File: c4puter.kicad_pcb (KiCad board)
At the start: 6 copper layers, 200 x 200 mm, 154 parts, among them J7 19V 3A, J8 DEBUG, Q1 DMN3016LDN, U1 ADP5054, U2 INA199, U3 AOZ1037, U5 INA199, U6 INA199, U8 INA199, U9 TLV70225DBV

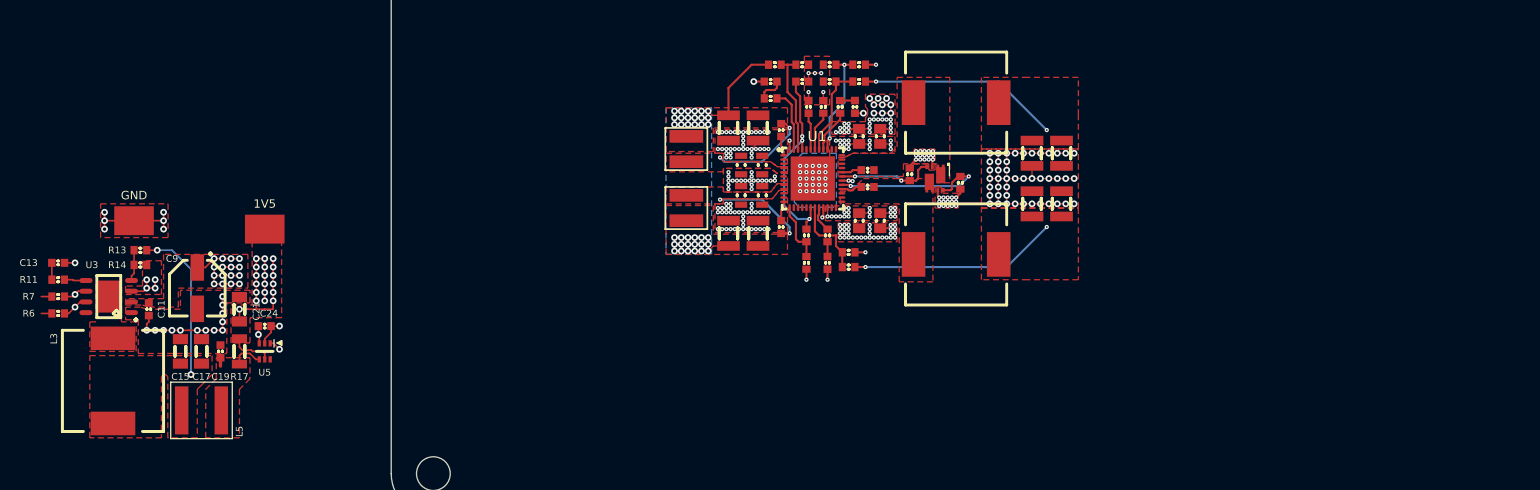
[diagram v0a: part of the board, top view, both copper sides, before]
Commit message: More power supply work
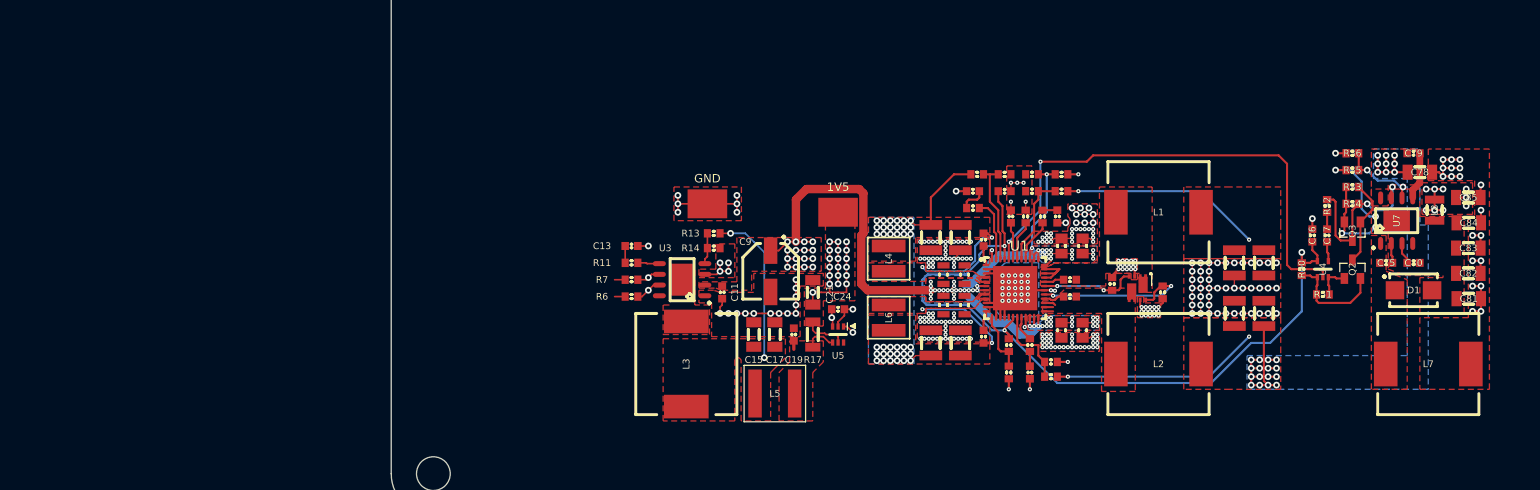
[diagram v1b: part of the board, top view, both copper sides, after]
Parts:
- added C75: 100n, IPC7351-Nominal:CAPC1608X55, F.Cu at (118.0, 170.0)
- added C76: 100n, IPC7351-Nominal:CAPC1608X55, F.Cu at (109.2, 166.8)
- added C77: 2n2, IPC7351-Nominal:CAPC1608X55, F.Cu at (111.0, 166.8)
- added C78: 22u, IPC7351-Nominal:CAPC3216X70, F.Cu at (122.0, 159.2)
- added C79: 100n, IPC7351-Nominal:CAPC1608X55, F.Cu at (121.2, 157.0)
- added C80: 1u, IPC7351-Nominal:CAPC1608X55, F.Cu at (121.2, 170.0)
- added C81: 22u, IPC7351-Nominal:CAPC3216X70, F.Cu at (127.8, 174.2)
- added C82: 22u, IPC7351-Nominal:CAPC3216X70, F.Cu at (127.8, 171.2)
- added C83: 22u, IPC7351-Nominal:CAPC3216X70, F.Cu at (127.8, 168.2)
- added C84: 22u, IPC7351-Nominal:CAPC3216X70, F.Cu at (127.8, 165.2)
- added C85: 22u, IPC7351-Nominal:CAPC3216X70, F.Cu at (127.8, 162.2)
- added D1: MBRS360B, IPC7351-Nominal:DIOM5436X244, F.Cu at (121.2, 173.2)
- added L7: 22u, manuf:BOURNS-SRR1210, F.Cu at (123.0, 182.0)
- added L8: 2u2, IPC7351-Nominal:INDC2520X220, F.Cu at (123.8, 163.8)
- added Q2: BSS84, smd-semi:SOT-23, F.Cu at (114.0, 170.8)
- added Q3: 2N7002, smd-semi:SOT-23, F.Cu at (114.0, 166.2)
- added R50: 10k, IPC7351-Nominal:RESC1608X50, F.Cu at (108.0, 170.8)
- added R51: 20k, IPC7351-Nominal:RESC1608X50, F.Cu at (110.5, 173.8)
- added R52: 1k, IPC7351-Nominal:RESC1608X50, F.Cu at (111.0, 163.2)
- added R53: 100k, IPC7351-Nominal:RESC1608X50, F.Cu at (114.0, 161.0)
- added R54: 100k, IPC7351-Nominal:RESC1608X50, F.Cu at (114.0, 163.0)
- added R55: 10k, IPC7351-Nominal:RESC1608X50, F.Cu at (114.0, 159.0)
- added R56: 10k, IPC7351-Nominal:RESC1608X50, F.Cu at (114.0, 157.0)
- added U4: 74HCT1G02, smd-semi:SC-70-5, F.Cu at (110.5, 170.8)
- added U7: RT7258GSP, IPC7351-Nominal:SOIC127P600X170-9, F.Cu at (119.2, 165.0)
- moved C11 68.0 mm to (39.2, 173.5)
- moved C13 68.0 mm to (28.5, 168.0)
- moved C15 68.0 mm to (43.0, 178.5)
- moved C17 68.0 mm to (45.5, 178.5)
- moved C19 68.0 mm to (47.8, 178.5)
- moved C21 68.0 mm to (50.0, 173.5)
- moved C24 68.0 mm to (53.0, 175.5)
- moved C9 68.0 mm to (45.0, 171.0)
- moved L3 68.0 mm to (35.0, 182.0)
- moved L5 68.0 mm to (45.5, 185.5)
- moved R11 68.0 mm to (28.5, 170.0)
- moved R13 68.0 mm to (38.2, 166.5)
- moved R14 68.0 mm to (38.2, 168.2)
- moved R17 68.0 mm to (50.0, 178.5)
- moved R6 68.0 mm to (28.5, 174.0)
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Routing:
- net /Power/VREG: track 23.9 -> 91.2 mm
- net +12: track 51.0 -> 113.2 mm
- net Net-(U1-Pad44): track 0.00 -> 60.3 mm, vias 0 -> 2
- net GND: track 278.8 -> 335.8 mm, vias 339 -> 360
- net P5V: track 24.7 -> 56.5 mm, vias 2 -> 27
- net /Power/UNFN12: track 0.00 -> 25.8 mm, vias 0 -> 4
- net Net-(Q3-Pad3): track 0.00 -> 20.1 mm, vias 0 -> 2
- net ENN12#: track 0.00 -> 12.3 mm
- net Net-(Q2-Pad3): track 0.00 -> 10.3 mm
- net N5V: track 0.00 -> 9.70 mm, vias 0 -> 9
- net Net-(R55-Pad1): track 0.00 -> 9.43 mm, vias 0 -> 2
- net /Power/SW3V: track 0.00 -> 5.67 mm
- net /Power/SW5V: track 0.00 -> 3.50 mm
- net /Power/SWA1V2: track 11.8 -> 14.6 mm
- net Net-(C80-Pad1): track 0.00 -> 2.55 mm
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- added copper zone on B.Cu, net +12
- added copper zone on F.Cu, net /Power/SWN12
- added copper zone on F.Cu, net /Power/UNFN12
- added copper zone on F.Cu, net N5V
- added copper zone on B.Cu, net P5V

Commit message: Uh, more misc work.
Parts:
- removed C10: 10u, IPC7351-Nominal:CAPC2012X70
- removed C11, C19, C22, C23, C24, C25, C26, C27, C32, C75, C76, C79: 100n, IPC7351-Nominal:CAPC1608X55
- removed C12, C16, C30, C31, C55, C56, C57, C59: 100u, IPC7351-Nominal:CAPC3225X88
- removed C13: 220p, IPC7351-Nominal:CAPC1608X55
- removed C14: 4n5, IPC7351-Nominal:CAPC1608X55
- removed C15, C17, C21, C78, C81, C82, C83, C84, C85: 22u, IPC7351-Nominal:CAPC3216X70
- removed C18: 3n6, IPC7351-Nominal:CAPC1608X55
- removed C20: 4n9, IPC7351-Nominal:CAPC1608X55
- removed C28, C29, C80: 1u, IPC7351-Nominal:CAPC1608X55
- removed C33, C34: 2u2, IPC7351-Nominal:CAPC1608X55
- removed C77: 2n2, IPC7351-Nominal:CAPC1608X55
- removed C9: 22u(P), IPC7351-Nominal:CAPAE660X570
- removed D1: MBRS360B, IPC7351-Nominal:DIOM5436X244
- removed L1, L2, L3: 4u7, manuf:BOURNS-SRR1210
- removed L4, L6: 6u8, manuf:BOURNS-SRN5040
- removed L5: 2u2, manuf:MURATA-DG6050C
- removed L7: 22u, manuf:BOURNS-SRR1210
- removed L8: 2u2, IPC7351-Nominal:INDC2520X220
- removed R56: 10k, IPC7351-Nominal:RESC1608X50
- removed TP3: 1V5, manuf:TESTPOINT-KEYSTONE-5018
- removed TP5: 2V5, manuf:TESTPOINT-KEYSTONE-5018
- removed TP6, TP7, TP8: GND, manuf:TESTPOINT-KEYSTONE-5018
- removed U2, U5, U6, U8: INA199, smd-semi:SC-70-6
- removed U3: AOZ1037, IPC7351-Nominal:SOIC127P600X175-9
- removed U4: 74HCT1G02, smd-semi:SC-70-5
- removed U7: RT7258GSP, IPC7351-Nominal:SOIC127P600X170-9
- removed U9: TLV70225DBV, smd-semi:SOT-23-5
- added DS1: PCI_P12(R), smd-semi:LED-0603, F.Cu at (86.5, 164.0)
- added DS10: BRG_P3V3(R), smd-semi:LED-0603, F.Cu at (96.5, 169.0)
- added DS11: CPU_P3V3(R), smd-semi:LED-0603, F.Cu at (96.5, 179.0)
- added DS12: AUX_P3V3(R), smd-semi:LED-0603, F.Cu at (96.5, 184.0)
- added DS13: SBY_P3V3(R), smd-semi:LED-0603, F.Cu at (96.5, 189.0)
- added DS14: PCI_P3V3(G), smd-semi:LED-0603, F.Cu at (98.5, 164.0)
- added DS15: BRG_P3V3(G), smd-semi:LED-0603, F.Cu at (98.5, 169.0)
- added DS16: CPU_P3V3(G), smd-semi:LED-0603, F.Cu at (98.5, 179.0)
- added DS17: AUX_P3V3(G), smd-semi:LED-0603, F.Cu at (98.5, 184.0)
- added DS18: SBY_P3V3(G), smd-semi:LED-0603, F.Cu at (98.5, 189.0)
- added DS19: BRG_P2V5(R), smd-semi:LED-0603, F.Cu at (101.5, 169.0)
- added DS2: PCI_P12(G), smd-semi:LED-0603, F.Cu at (88.5, 164.0)
- added DS20: CPU_P2V5(R), smd-semi:LED-0603, F.Cu at (101.5, 179.0)
- added DS21: BRG_P2V5(G), smd-semi:LED-0603, F.Cu at (103.5, 169.0)
- added DS22: CPU_P2V5(G), smd-semi:LED-0603, F.Cu at (103.5, 179.0)
- added DS23: BRG_P1V5(R), smd-semi:LED-0603, F.Cu at (106.5, 169.0)
- added DS24: MEM_P1V5(R), smd-semi:LED-0603, F.Cu at (106.5, 174.0)
- added DS25: CPU_P1V5(R), smd-semi:LED-0603, F.Cu at (106.5, 179.0)
- added DS26: BRG_P1V5(G), smd-semi:LED-0603, F.Cu at (108.5, 169.0)
- added DS27: MEM_P1V5(G), smd-semi:LED-0603, F.Cu at (108.5, 174.0)
- added DS28: CPU_P1V5(G), smd-semi:LED-0603, F.Cu at (108.5, 179.0)
- added DS29: BRG_P1V2(R), smd-semi:LED-0603, F.Cu at (111.5, 169.0)
- added DS3: PCI_P5(R), smd-semi:LED-0603, F.Cu at (91.5, 164.0)
- added DS30: CPU_P1V2(R), smd-semi:LED-0603, F.Cu at (111.5, 179.0)
- added DS31: BRG_P1V2(G), smd-semi:LED-0603, F.Cu at (113.5, 169.0)
- added DS32: CPU_P1V2(G), smd-semi:LED-0603, F.Cu at (113.5, 179.0)
- added DS33: PCI_N12(R), smd-semi:LED-0603, F.Cu at (116.5, 164.0)
- added DS34: MEM_PV75(R), smd-semi:LED-0603, F.Cu at (116.5, 174.0)
- added DS35: PCI_N12(G), smd-semi:LED-0603, F.Cu at (118.5, 164.0)
- added DS36: MEM_PV75(G), smd-semi:LED-0603, F.Cu at (118.5, 174.0)
- added DS37: POWER(R), smd-semi:LED-0603, F.Cu at (135.0, 164.0)
- added DS38: CARD(R), smd-semi:LED-0603, F.Cu at (135.0, 169.0)
- added DS39: BIT(R), smd-semi:LED-0603, F.Cu at (135.0, 174.0)
- added DS4: BRG_P5(R), smd-semi:LED-0603, F.Cu at (91.5, 169.0)
- added DS40: CLK(R), smd-semi:LED-0603, F.Cu at (135.0, 179.0)
- added DS41: MEM(R), smd-semi:LED-0603, F.Cu at (135.0, 184.0)
- added DS42: RUN(R), smd-semi:LED-0603, F.Cu at (135.0, 189.0)
- added DS43: POWER(G), smd-semi:LED-0603, F.Cu at (137.0, 164.0)
- added DS44: CARD(G), smd-semi:LED-0603, F.Cu at (137.0, 169.0)
- added DS45: BIT-BR(G), smd-semi:LED-0603, F.Cu at (137.0, 174.0)
- added DS46: CLK(G), smd-semi:LED-0603, F.Cu at (137.0, 179.0)
- added DS47: MEM(G), smd-semi:LED-0603, F.Cu at (137.0, 184.0)
- added DS48: RUN(G), smd-semi:LED-0603, F.Cu at (137.0, 189.0)
- added DS49: BIT-CPU0(G), smd-semi:LED-0603, F.Cu at (145.5, 174.0)
- added DS5: CPU_P5(R), smd-semi:LED-0603, F.Cu at (91.5, 179.0)
- added DS50: BIT-CPU1(G), smd-semi:LED-0603, F.Cu at (152.5, 174.0)
- added DS51: UPDOG(G), smd-semi:LED-0603, F.Cu at (151.0, 189.0)
- added DS52: UNC(R), smd-semi:LED-0603, F.Cu at (161.5, 164.0)
- added DS53: UNC(R), smd-semi:LED-0603, F.Cu at (161.5, 169.0)
- added DS54: UNC(R), smd-semi:LED-0603, F.Cu at (161.5, 174.0)
- added DS55: UNC(R), smd-semi:LED-0603, F.Cu at (161.5, 179.0)
- added DS56: UNC(R), smd-semi:LED-0603, F.Cu at (161.5, 184.0)
- added DS57: UNC(R), smd-semi:LED-0603, F.Cu at (161.5, 189.0)
- added DS58: UNC(G), smd-semi:LED-0603, F.Cu at (163.5, 164.0)
- added DS59: UNC(G), smd-semi:LED-0603, F.Cu at (163.5, 169.0)
- added DS6: PCI_P5(G), smd-semi:LED-0603, F.Cu at (93.5, 164.0)
- added DS60: UNC(G), smd-semi:LED-0603, F.Cu at (163.5, 174.0)
- added DS61: UNC(G), smd-semi:LED-0603, F.Cu at (163.5, 179.0)
- added DS62: UNC(G), smd-semi:LED-0603, F.Cu at (163.5, 184.0)
- added DS63: UNC(G), smd-semi:LED-0603, F.Cu at (163.5, 189.0)
- added DS7: BRG_P5(G), smd-semi:LED-0603, F.Cu at (93.5, 169.0)
- added DS8: CPU_P5(G), smd-semi:LED-0603, F.Cu at (93.5, 179.0)
- added DS9: PCI_P3V3(R), smd-semi:LED-0603, F.Cu at (96.5, 164.0)
- added DZ1: DRTR5V0U2SR, smd-semi:SOT-143, F.Cu at (21.2, 10.0)
- added J1: PDI, conn-100mil:CONN-100MIL-M-2x3, F.Cu at (157.0, 153.5)
- added PSU1: C4-0-PSU, conn-fci:CONN-10018783-10202TLF-PCIEx8-FCI, F.Cu at (33.0, 182.0)
- C1: value 10u -> 1u
- C2, C7: value 10u -> 100n; footprint IPC7351-Nominal:CAPC2012X70 -> IPC7351-Nominal:CAPC1005X55
- C3, C4, C5, C6: value 10u -> 390u; footprint IPC7351-Nominal:CAPC2012X70 -> pth-passive:C-ALUM-8mm
- C8: footprint IPC7351-Nominal:CAPC1608X55 -> IPC7351-Nominal:CAPC1005X55
- CPU0, CPU1: value XC6SLX16-2FTG256C -> XC6SLX25-FGG484; footprint manuf:XILINX-FT256 -> manuf:XILINX-FGG484
- LIMB1: value ATSAME70NnnA-AN -> LPC435xFET256; footprint IPC7351-Nominal:QFP50P1600X1600X160-100 -> smd-semi:BGA100P1700X1700-256
- Q1: value DMN3016LDN -> AOD4189; footprint manuf:DIODES-V-DFN3030-8 -> smd-semi:TO-252
- Q2: value BSS84 -> AOD4189; footprint smd-semi:SOT-23 -> smd-semi:TO-252
- R1: value 30k -> 100k
- R10: value 38k5 -> 750
- R11: value 10k -> 300
- R12: value 22k -> 300
- R13, R50: value 10k -> 750
- R14, R55: value 10k -> 51k
- R15: value 22k -> 750
- R16, R18, R21: value R-0603 -> 300
- R17: value 0R005 -> 51k; footprint IPC7351-Nominal:RESC3216X60 -> IPC7351-Nominal:RESC1608X50
- R19, R20: value R-0603 -> 750
- R2: value 100k -> 330k
- R22: value R-0603 -> 51k
- R3: value 10k -> 100k
- R4: value 500k -> 10k
- R5: value 200k -> 750
- R51: value 20k -> 750
- R52: value 1k -> 51k
- R53, R54, R6: value 100k -> 300
- R7: value 100k -> 51k
- R8: value 8k6 -> 51k
- R9: value 7k8 -> 51k
- U1: value ADP5054 -> ATXMEGA8E5-MU; footprint IPC7351-Nominal:QFN50P700X700X80-49 -> IPC7351-Nominal:QFN50P500X500X100-33
- moved Q3 175.1 mm to (43.5, 6.00), turned to 90 degrees
- moved R4 170.9 mm to (43.5, 11.5), turned to 180 degrees
- moved R11 162.1 mm to (190.0, 155.5), turned to 90 degrees
- moved R6 154.2 mm to (181.0, 151.5), turned to 270 degrees
- moved R3 153.5 mm to (43.5, 9.50), turned to 180 degrees
- moved R13 151.5 mm to (189.0, 151.5), turned to 90 degrees
- moved R7 123.9 mm to (151.0, 153.5), turned to 270 degrees
- moved C8 117.0 mm to (163.2, 149.4)
- moved R21 113.3 mm to (186.0, 155.5), turned to 90 degrees
- moved R19 112.9 mm to (187.0, 151.5), turned to 90 degrees
- moved R5 112.2 mm to (182.0, 155.5), turned to 270 degrees
- moved R16 112.2 mm to (188.0, 155.5), turned to 90 degrees
- moved R10 111.3 mm to (180.0, 155.5), turned to 90 degrees
- moved Q2 108.3 mm to (17.0, 122.5), turned to 180 degrees
- moved C7 107.3 mm to (171.6, 155.6), turned to 270 degrees
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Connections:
- C1 pad 1: +12 -> Net-(C1-Pad1)
- C1 pad 2: GND -> Net-(C1-Pad2)
- C2 pad 2: GND -> Net-(C1-Pad2)
- C7 pad 1: +12 -> GND
- C7 pad 2: GND -> SBY_P3V3
- C8 pad 1: +3.3SB -> GND
- C8 pad 2: GND -> SBY_P3V3
- CPU0 pad A15: (no net) -> Net-(CPU0-PadA15)
- CPU0 pad A16: (no net) -> Net-(CPU0-PadA16)
- CPU0 pad A3: (no net) -> Net-(CPU0-PadA3)
- CPU0 pad B11: (no net) -> Net-(CPU0-PadB11)
- CPU0 pad B15: (no net) -> Net-(CPU0-PadB15)
- CPU0 pad B16: (no net) -> Net-(CPU0-PadB16)
- CPU0 pad B4: (no net) -> Net-(CPU0-PadB4)
- CPU0 pad B5: Net-(CPU0-PadB5) -> (no net)
- CPU0 pad B7: (no net) -> Net-(CPU0-PadB7)
- CPU0 pad C12: (no net) -> Net-(CPU0-PadC12)
- CPU0 pad C14: (no net) -> Net-(CPU0-PadC14)
- CPU0 pad C15: (no net) -> Net-(CPU0-PadC15)
- CPU0 pad C16: (no net) -> Net-(CPU0-PadC16)
- CPU0 pad C4: Net-(CPU0-PadC4) -> (no net)
- CPU0 pad D10: (no net) -> Net-(CPU0-PadD10)
- CPU0 pad D13: (no net) -> Net-(CPU0-PadD13)
- CPU0 pad D14: (no net) -> Net-(CPU0-PadD14)
- CPU0 pad D15: (no net) -> Net-(CPU0-PadD15)
- CPU0 pad D5: Net-(CPU0-PadD5) -> (no net)
- CPU0 pad D7: (no net) -> Net-(CPU0-PadD7)
- CPU0 pad E10: Net-(CPU0-PadE10) -> (no net)
- CPU0 pad E11: Net-(CPU0-PadE11) -> (no net)
- CPU0 pad E12: (no net) -> Net-(CPU0-PadE12)
- CPU0 pad E13: (no net) -> Net-(CPU0-PadE13)
- CPU0 pad E14: (no net) -> Net-(CPU0-PadE14)
- CPU0 pad E16: (no net) -> Net-(CPU0-PadE16)
- CPU0 pad E6: Net-(CPU0-PadE6) -> (no net)
- CPU0 pad E7: Net-(CPU0-PadE7) -> (no net)
- CPU0 pad E8: Net-(CPU0-PadE8) -> (no net)
- CPU0 pad E9: (no net) -> Net-(CPU0-PadE9)
- CPU0 pad F10: Net-(CPU0-PadF10) -> (no net)
- CPU0 pad F12: (no net) -> Net-(CPU0-PadF12)
- CPU0 pad F13: (no net) -> Net-(CPU0-PadF13)
- CPU0 pad F14: (no net) -> Net-(CPU0-PadF14)
- CPU0 pad F15: (no net) -> Net-(CPU0-PadF15)
- CPU0 pad F7: Net-(CPU0-PadF7) -> (no net)
- CPU0 pad F9: Net-(CPU0-PadF9) -> (no net)
- CPU0 pad G10: (no net) -> Net-(CPU0-PadG10)
- CPU0 pad G13: (no net) -> Net-(CPU0-PadG13)
- CPU0 pad G14: (no net) -> Net-(CPU0-PadG14)
- CPU0 pad H12: (no net) -> Net-(CPU0-PadH12)
- CPU0 pad H13: (no net) -> Net-(CPU0-PadH13)
- CPU0 pad H14: (no net) -> Net-(CPU0-PadH14)
- CPU1 pad A15: (no net) -> Net-(CPU1-PadA15)
- CPU1 pad A16: (no net) -> Net-(CPU1-PadA16)
- CPU1 pad A3: (no net) -> Net-(CPU1-PadA3)
- CPU1 pad B11: (no net) -> Net-(CPU1-PadB11)
- CPU1 pad B15: (no net) -> Net-(CPU1-PadB15)
- CPU1 pad B16: (no net) -> Net-(CPU1-PadB16)
- CPU1 pad B4: (no net) -> Net-(CPU1-PadB4)
- CPU1 pad B5: Net-(CPU1-PadB5) -> (no net)
- CPU1 pad B7: (no net) -> Net-(CPU1-PadB7)
- CPU1 pad C12: (no net) -> Net-(CPU1-PadC12)
- CPU1 pad C14: (no net) -> Net-(CPU1-PadC14)
- CPU1 pad C15: (no net) -> Net-(CPU1-PadC15)
- CPU1 pad C16: (no net) -> Net-(CPU1-PadC16)
- CPU1 pad C4: Net-(CPU1-PadC4) -> (no net)
- CPU1 pad D10: (no net) -> Net-(CPU1-PadD10)
- CPU1 pad D13: (no net) -> Net-(CPU1-PadD13)
- CPU1 pad D14: (no net) -> Net-(CPU1-PadD14)
- CPU1 pad D15: (no net) -> Net-(CPU1-PadD15)
- CPU1 pad D5: Net-(CPU1-PadD5) -> (no net)
- CPU1 pad D7: (no net) -> Net-(CPU1-PadD7)
- CPU1 pad E10: Net-(CPU1-PadE10) -> (no net)
- CPU1 pad E11: Net-(CPU1-PadE11) -> (no net)
- CPU1 pad E12: (no net) -> Net-(CPU1-PadE12)
- CPU1 pad E13: (no net) -> Net-(CPU1-PadE13)
- CPU1 pad E14: (no net) -> Net-(CPU1-PadE14)
- CPU1 pad E16: (no net) -> Net-(CPU1-PadE16)
- CPU1 pad E6: Net-(CPU1-PadE6) -> (no net)
- CPU1 pad E7: Net-(CPU1-PadE7) -> (no net)
- CPU1 pad E8: Net-(CPU1-PadE8) -> (no net)
- CPU1 pad E9: (no net) -> Net-(CPU1-PadE9)
- CPU1 pad F10: Net-(CPU1-PadF10) -> (no net)
- CPU1 pad F12: (no net) -> Net-(CPU1-PadF12)
- CPU1 pad F13: (no net) -> Net-(CPU1-PadF13)
- CPU1 pad F14: (no net) -> Net-(CPU1-PadF14)
- CPU1 pad F15: (no net) -> Net-(CPU1-PadF15)
- CPU1 pad F7: Net-(CPU1-PadF7) -> (no net)
- CPU1 pad F9: Net-(CPU1-PadF9) -> (no net)
- CPU1 pad G10: (no net) -> Net-(CPU1-PadG10)
- CPU1 pad G13: (no net) -> Net-(CPU1-PadG13)
- CPU1 pad G14: (no net) -> Net-(CPU1-PadG14)
- CPU1 pad H12: (no net) -> Net-(CPU1-PadH12)
- CPU1 pad H13: (no net) -> Net-(CPU1-PadH13)
- CPU1 pad H14: (no net) -> Net-(CPU1-PadH14)
- J7 pad 1: V+ -> /12VIN
- J8 pad 1: Net-(J8-Pad1) -> Net-(DZ1-Pad4)
- J8 pad 2: Net-(J8-Pad2) -> /EC/USB0_D+
- J8 pad 3: Net-(J8-Pad3) -> /EC/USB0_D-
- J8 pad 5: Net-(J8-Pad5) -> GND
- J8 pad SH: Net-(J8-PadSH) -> GND
- Q1 pad 1: /Power/SW3V -> Net-(C1-Pad2)
- Q1 pad 2: GND -> Net-(C1-Pad1)
- Q1 pad 3: Net-(Q1-Pad3) -> /12VIN
- Q2 pad 1: GND -> Net-(C1-Pad2)
- Q2 pad 2: ENN12# -> Net-(C1-Pad1)
- Q2 pad 3: Net-(Q2-Pad3) -> +12
- Q3 pad 1: Net-(Q2-Pad3) -> Net-(DZ1-Pad4)
- Q3 pad 2: /Power/UNFN12 -> Net-(Q3-Pad2)
- Q3 pad 3: Net-(Q3-Pad3) -> 3V3_LIMB
- R1 pad 1: GND -> Net-(C1-Pad2)
- R1 pad 2: Net-(R1-Pad2) -> GND
- R10 pad 1: Net-(R10-Pad1) -> /Blinkenlights/COL0
- R10 pad 2: Net-(C20-Pad1) -> Net-(R10-Pad2)
- R11 pad 1: Net-(R11-Pad1) -> /Blinkenlights/COL6
- R11 pad 2: Net-(C13-Pad1) -> Net-(R11-Pad2)
- R12 pad 1: Net-(Q1-Pad3) -> /Blinkenlights/COL1
- R12 pad 2: GND -> Net-(R12-Pad2)
- R13 pad 1: Net-(R13-Pad1) -> /Blinkenlights/COL7
- R13 pad 2: /Power/RAW1V5 -> Net-(R13-Pad2)
- R14 pad 1: GND -> SBY_P3V3
- R14 pad 2: Net-(R13-Pad1) -> /Blinkenlights/ROW2
- R15 pad 1: Net-(Q1-Pad6) -> /Blinkenlights/COL2
- R15 pad 2: GND -> Net-(R15-Pad2)
- R16 pad 1: Net-(R16-Pad1) -> /Blinkenlights/COL8
- R16 pad 2: GND -> Net-(R16-Pad2)
- R17 pad 1: /Power/1V5 -> SBY_P3V3
- R17 pad 2: /Power/S+1V5 -> /Blinkenlights/ROW3
- R18 pad 1: P3V -> /Blinkenlights/COL3
- R18 pad 2: Net-(R16-Pad1) -> Net-(R18-Pad2)
- R19 pad 1: Net-(R19-Pad1) -> /Blinkenlights/COL9
- R19 pad 2: GND -> Net-(R19-Pad2)
- R2 pad 1: Net-(R2-Pad1) -> Net-(C1-Pad1)
- R2 pad 2: +12 -> Net-(C1-Pad2)
- R20 pad 1: P5V -> /Blinkenlights/COL4
- R20 pad 2: Net-(R19-Pad1) -> Net-(R20-Pad2)
- R21 pad 1: GND -> /Blinkenlights/COL10
- R22 pad 1: +1.2 -> SBY_P3V3
- R22 pad 2: Net-(R21-Pad2) -> /Blinkenlights/ROW4
- R3 pad 1: GND -> Net-(Q3-Pad2)
- R3 pad 2: Net-(R2-Pad1) -> GND
- R4 pad 1: Net-(R4-Pad1) -> /EC/USB0_VBUS
- R4 pad 2: /Power/VREG -> Net-(Q3-Pad2)
- R5 pad 1: GND -> Net-(R5-Pad1)
- R5 pad 2: Net-(R4-Pad1) -> /Blinkenlights/COL14
- R50 pad 1: /Power/VREG -> /Blinkenlights/COL5
- R50 pad 2: ENN12# -> Net-(R50-Pad2)
- R51 pad 1: ENN12# -> /Blinkenlights/COL11
- R51 pad 2: GND -> Net-(R51-Pad2)
- R52 pad 1: Net-(C77-Pad1) -> SBY_P3V3
- R52 pad 2: Net-(Q3-Pad3) -> /Blinkenlights/ROW5
- R53 pad 1: Net-(Q2-Pad3) -> /Blinkenlights/COL12
- R53 pad 2: /Power/UNFN12 -> Net-(R53-Pad2)
- R54 pad 1: Net-(Q3-Pad3) -> /Blinkenlights/COL13
- R54 pad 2: /Power/UNFN12 -> Net-(R54-Pad2)
- R55 pad 1: Net-(R55-Pad1) -> SBY_P3V3
- R55 pad 2: /Power/UNFN12 -> /Blinkenlights/ROW6
- R6 pad 1: +3.3SB -> Net-(R6-Pad1)
- R6 pad 2: /Power/PG1V5 -> /Blinkenlights/COL15
- R7 pad 1: /Power/EN1V5 -> SBY_P3V3
- R7 pad 2: GND -> Net-(J1-Pad5)
- R8 pad 1: Net-(R8-Pad1) -> SBY_P3V3
- R8 pad 2: Net-(C14-Pad1) -> /Blinkenlights/ROW0
- R9 pad 1: Net-(R9-Pad1) -> SBY_P3V3
- R9 pad 2: Net-(C18-Pad1) -> /Blinkenlights/ROW1
- U1 pad 1: Net-(C26-Pad2) -> GND
- U1 pad 10: GND -> Net-(R20-Pad2)
- U1 pad 11: GND -> Net-(R18-Pad2)
- U1 pad 12: Net-(C27-Pad2) -> Net-(R15-Pad2)
- U1 pad 13: Net-(R4-Pad1) -> Net-(R12-Pad2)
- U1 pad 14: GND -> Net-(R10-Pad2)
- U1 pad 15: GND -> /Blinkenlights/SCL
- U1 pad 16: GND -> /Blinkenlights/SDA
- U1 pad 17: Net-(U1-Pad17) -> SBY_P3V3
- U1 pad 18: /Power/VREG -> GND
- U1 pad 19: Net-(R19-Pad1) -> Net-(R6-Pad1)
- U1 pad 2: GND -> /Blinkenlights/ROW4
- U1 pad 20: Net-(R9-Pad1) -> Net-(R5-Pad1)
- U1 pad 21: Net-(U1-Pad21) -> Net-(R54-Pad2)
- U1 pad 22: +12 -> Net-(R53-Pad2)
- U1 pad 23: +12 -> Net-(R51-Pad2)
- U1 pad 24: +12 -> Net-(R21-Pad2)
- U1 pad 25: /Power/SW5V -> Net-(R19-Pad2)
- U1 pad 26: /Power/SW5V -> Net-(R16-Pad2)
- U1 pad 27: /Power/SW5V -> Net-(R13-Pad2)
- U1 pad 28: Net-(C25-Pad2) -> Net-(R11-Pad2)
- U1 pad 29: Net-(Q1-Pad6) -> /Blinkenlights/ROW7
- U1 pad 3: GND -> /Blinkenlights/ROW3
- U1 pad 30: GND -> /Blinkenlights/ROW6
- U1 pad 31: Net-(Q1-Pad3) -> /Blinkenlights/ROW5
- U1 pad 32: Net-(C22-Pad2) -> SBY_P3V3
- U1 pad 33: /Power/SW3V -> GND
- U1 pad 4: /Power/SWA1V2 -> /Blinkenlights/ROW2
- U1 pad 5: /Power/SWA1V2 -> /Blinkenlights/ROW1
- U1 pad 6: +12 -> /Blinkenlights/ROW0
- U1 pad 7: +12 -> Net-(J1-Pad1)
- U1 pad 8: /Power/SWB1V2 -> Net-(J1-Pad5)
- U1 pad 9: /Power/SWB1V2 -> Net-(R50-Pad2)
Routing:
- net GND: track 335.8 -> 84.2 mm, vias 360 -> 94
- net /Blinkenlights/ROW4: track 0.00 -> 201.2 mm, vias 0 -> 2
- net /Blinkenlights/ROW5: track 0.00 -> 199.6 mm
- net /Blinkenlights/COL1: track 0.00 -> 197.2 mm, vias 0 -> 5
- net /Blinkenlights/ROW3: track 0.00 -> 192.7 mm, vias 0 -> 2
- net /Blinkenlights/COL0: track 0.00 -> 191.6 mm, vias 0 -> 5
- net /Blinkenlights/COL3: track 0.00 -> 186.5 mm, vias 0 -> 6
- net /Blinkenlights/COL2: track 0.00 -> 184.7 mm, vias 0 -> 6
- net /Blinkenlights/COL5: track 0.00 -> 183.5 mm, vias 0 -> 4
- net /Blinkenlights/ROW2: track 0.00 -> 183.1 mm, vias 0 -> 2
- net /Blinkenlights/COL4: track 0.00 -> 177.1 mm, vias 0 -> 3
- net /Blinkenlights/ROW0: track 0.00 -> 170.5 mm, vias 0 -> 2
- net /Blinkenlights/ROW1: track 0.00 -> 169.1 mm, vias 0 -> 2
- net /12VIN: track 0.00 -> 158.9 mm, vias 0 -> 30
- net /Blinkenlights/COL6: track 0.00 -> 153.6 mm, vias 0 -> 6
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- added copper zone on B.Cu, net /12VIN
- added copper zone on F.Cu, net /12VIN
- removed copper zone on B.Cu, net +1.2
- removed copper zone on F.Cu, net +1.2
- removed copper zone on B.Cu, net +12
- removed copper zone on F.Cu, net /Power/1V5
- removed copper zone on F.Cu, net /Power/RAW1V5
- removed copper zone on F.Cu, net /Power/S+1V5
- removed copper zone on F.Cu, net /Power/SW1V5
- removed copper zone on F.Cu, net /Power/SW3V
- removed copper zone on F.Cu, net /Power/SW5V
- removed copper zone on F.Cu, net /Power/SWA1V2
- removed copper zone on F.Cu, net /Power/SWB1V2
- removed copper zone on F.Cu, net /Power/SWN12
- removed copper zone on F.Cu, net /Power/UNFN12
- removed copper zone on B.Cu, net GND
- removed copper zone on F.Cu, net GND
- removed copper zone on F.Cu, net N5V
- removed copper zone on F.Cu, net P3V
- removed copper zone on B.Cu, net P5V
- removed copper zone on F.Cu, net P5V
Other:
- net class Default: via_dia 0.5 -> 0.8; via_drill 0.2 -> 0.4
- board text added: "AUX"
- board text added: "BOOT SEQUENCE"
- board text added: "BRIDGE"
- board text added: "CARD"
- board text added: "CLOCK"
- board text added: "CPU"
- board text added: "CPU0"
- board text added: "CPU1"
- board text added: "FPGA BITST"
- board text added: "MEM LOAD"
- board text added: "N12"
- board text added: "P12"
- board text added: "P1V2"
- board text added: "P1V5"
- board text added: "P2V5"
- board text added: "P3V3"
- board text added: "P5"
- board text added: "PCI"
- board text added: "POWER SEQ"
- board text added: "PV75"
- board text added: "RUN"
- board text added: "SDRAM"
- board text added: "STBY"
- board text added: "UPDOG"
- board text added: "misc"
